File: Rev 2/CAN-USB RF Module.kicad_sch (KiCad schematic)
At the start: 37 parts, among them IC1 ESDALC6V1W5, J1 Conn_02x05_Top_Bottom, J5 Conn_Coaxial, SW1 RESET, SW2 BOOT0, SW3 GPSW, U1 8MHz, U2 STM32L432KBU6

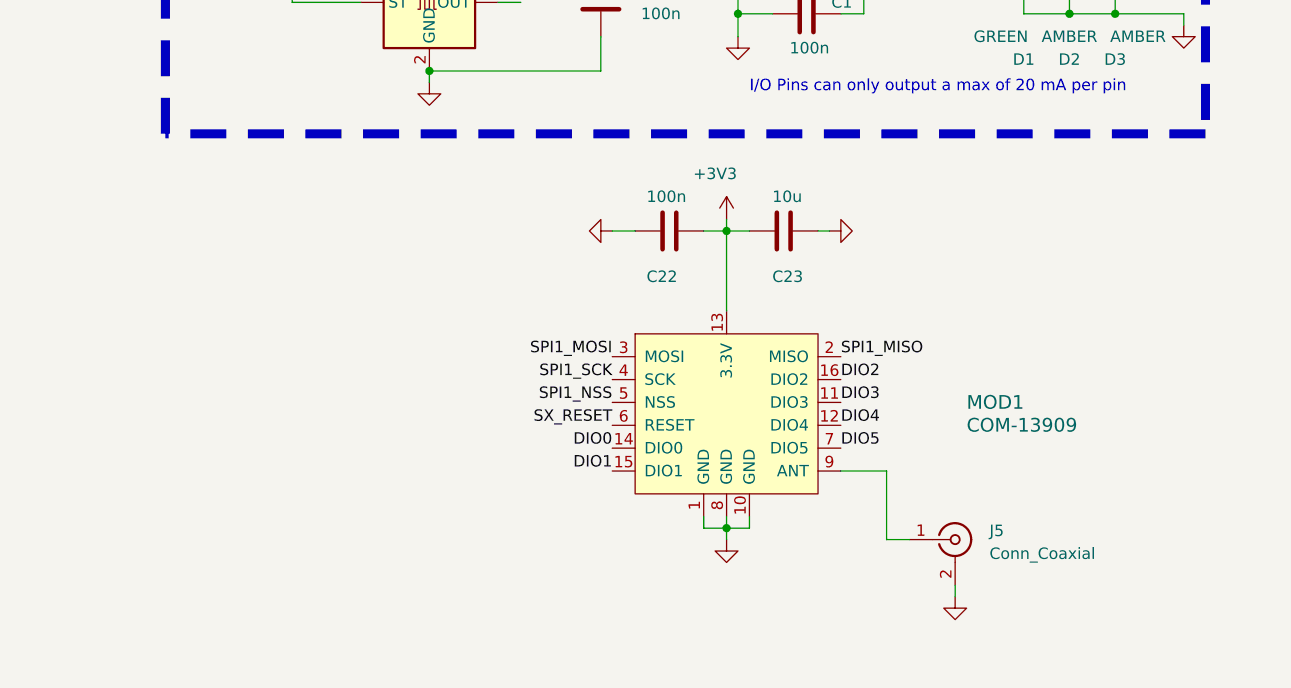
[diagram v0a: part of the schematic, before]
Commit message: Thats it no more changes
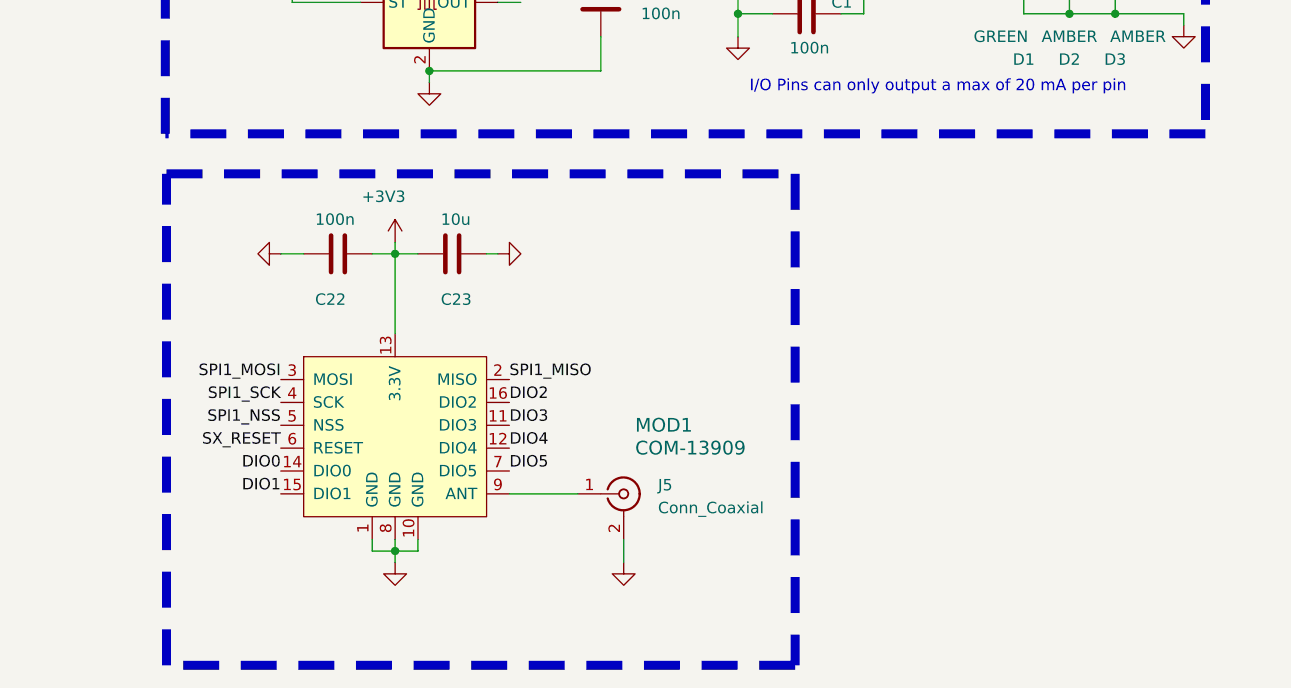
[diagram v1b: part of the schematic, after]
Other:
- moved on the sheet: C22, C23, J5, MOD1
